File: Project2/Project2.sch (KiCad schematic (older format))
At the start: 75 parts

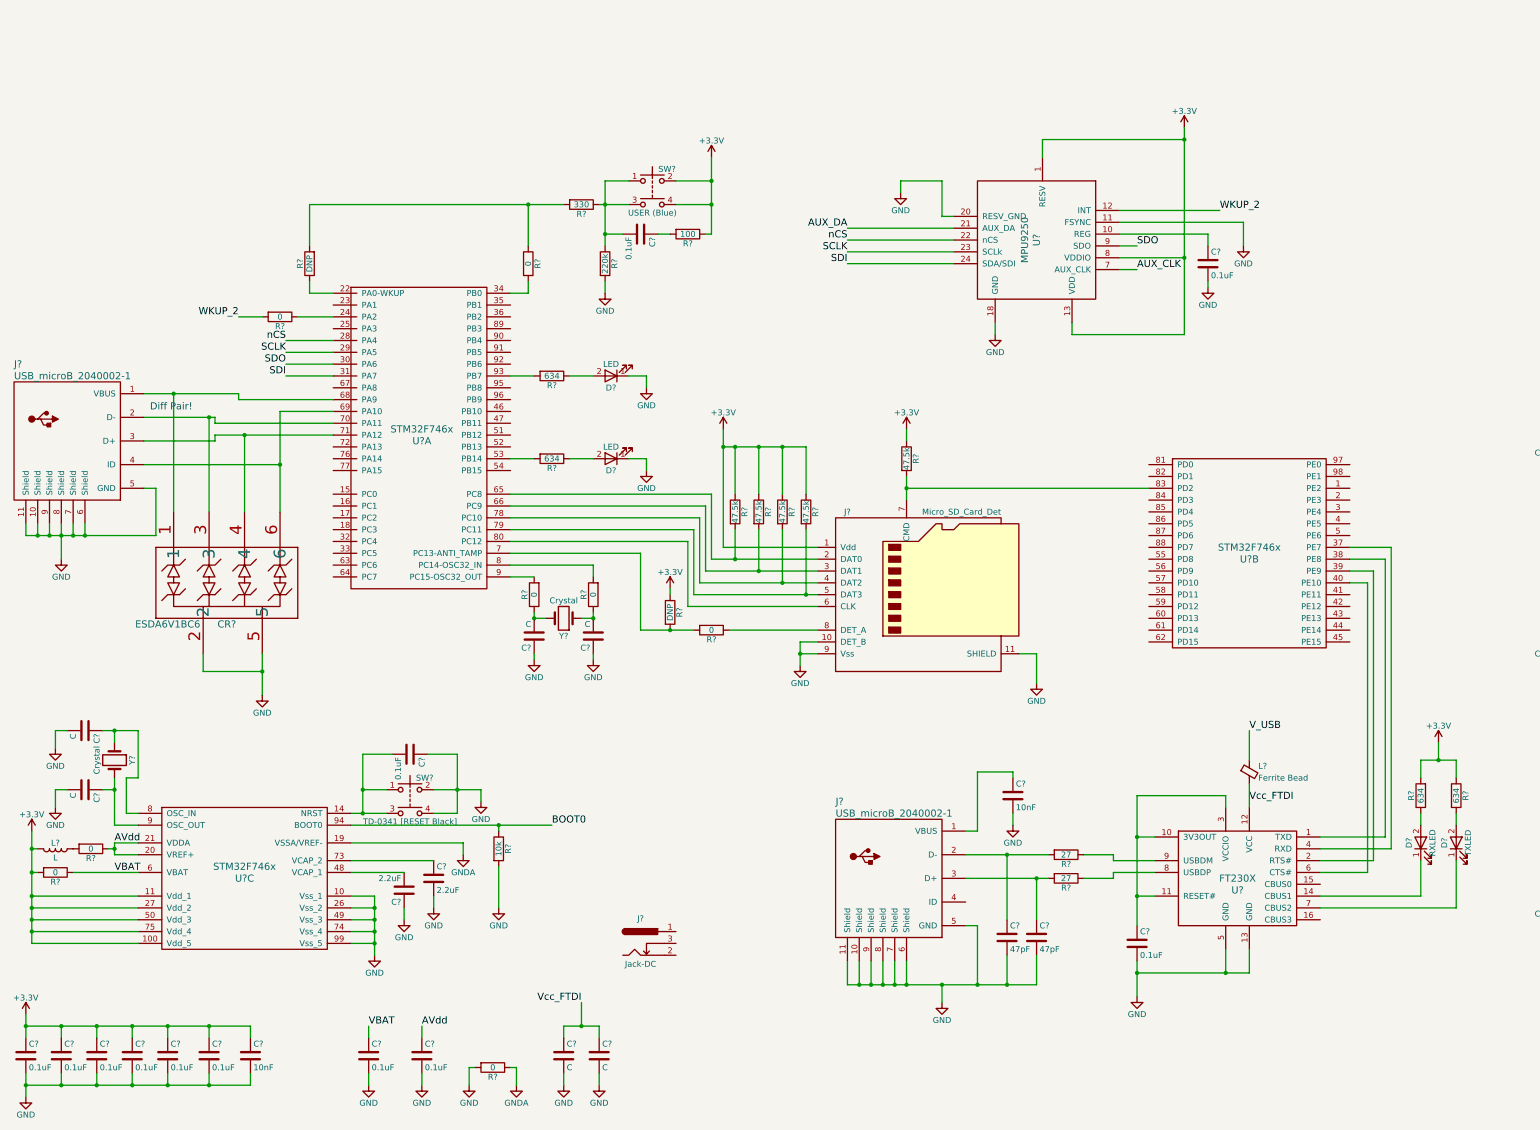
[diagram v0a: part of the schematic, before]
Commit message: Made some updates
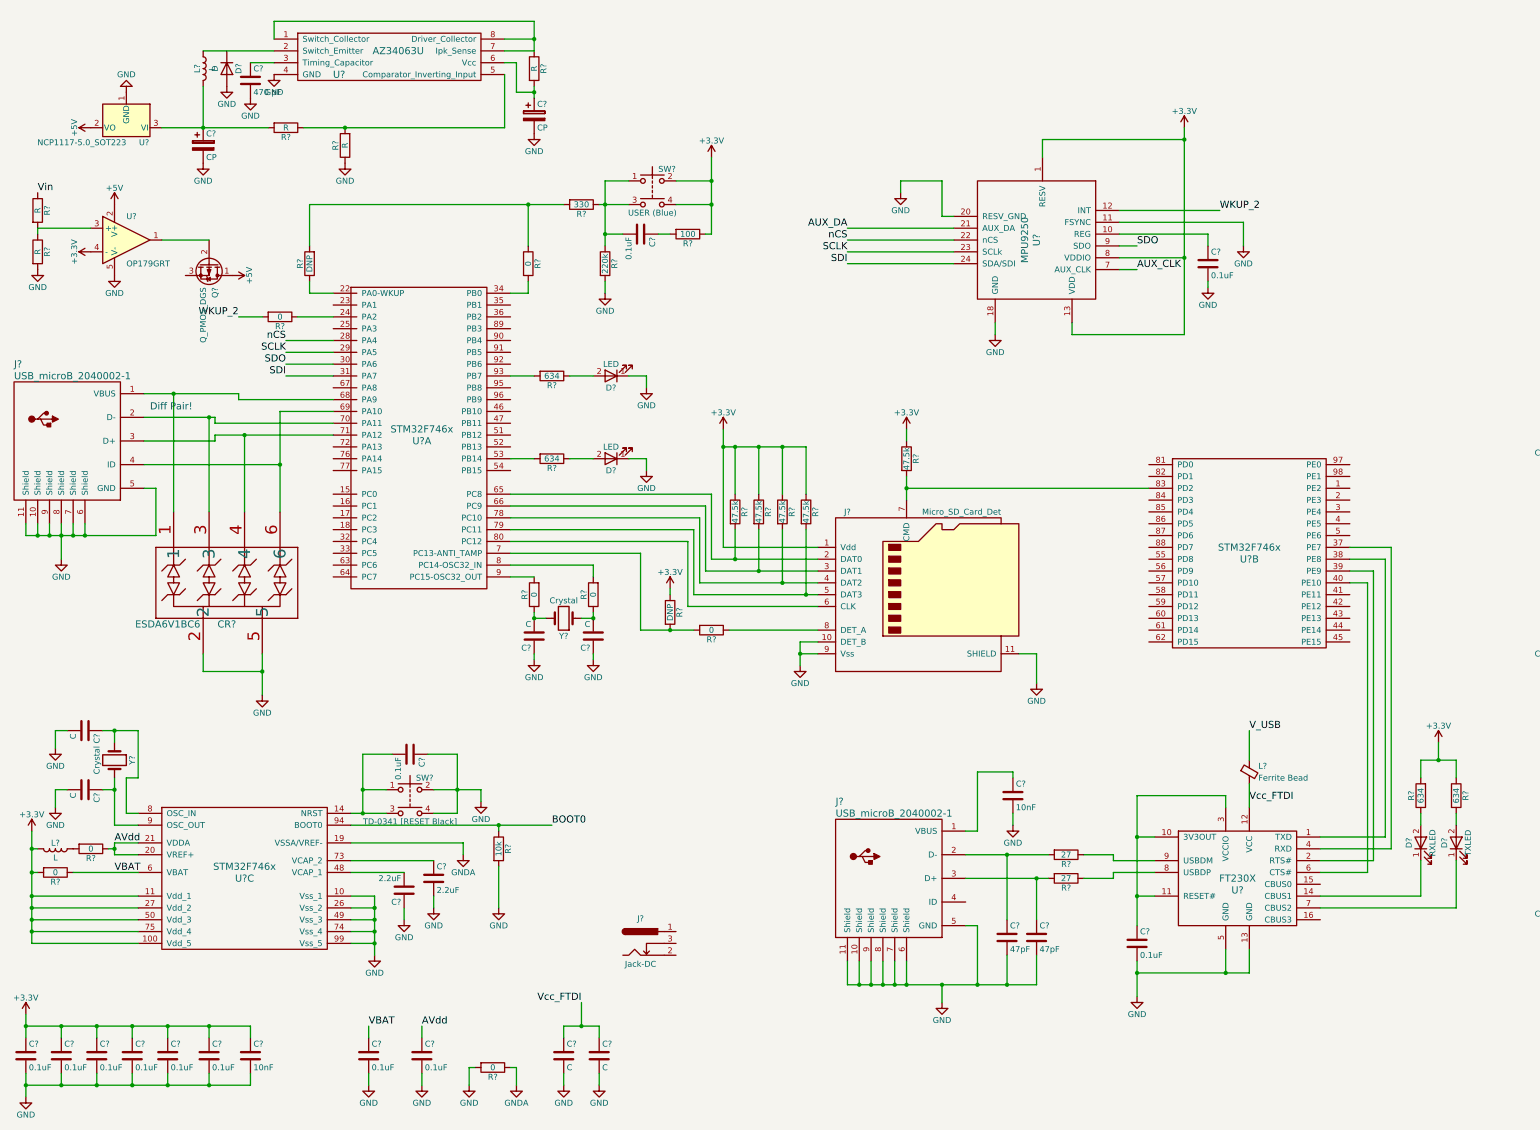
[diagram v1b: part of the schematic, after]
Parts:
- added C?: 470 pF, symbol C
- added C? (x2): CP, symbol CP
- added D?: D, symbol D
- added L?: L, symbol L
- added Q?: Q_PMOS_DGS, symbol Q_PMOS_DGS
- added R? (x5): R, symbol R
- added U?: AZ34063U, symbol AZ34063U
- added U?: NCP1117-5.0_SOT223, TO_SOT_Packages_SMD:SOT-223-3Lead_TabPin2, symbol NCP1117-5.0_SOT223
- added U?: OP179GRT, TO_SOT_Packages_SMD:SOT-23-5, symbol OP179GRT
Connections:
- net +3V3: now also U?.4 (-)
- net GND: now also C?.2, C?.2, C?.2, D?.2 (A), R?.1, R?.2, U?.1 (GND), U?.4 (GND), U?.5 (V-)
- new net: R?.1, U?.1 (Switch_Collector), U?.7 (Ipk_Sense), U?.8 (Driver_Collector)
- new net: L?.1, U?.2 (Switch_Emitter)
- new net: C?.1, U?.3 (Timing_Capacitor)
- new net: R?.1, R?.2, U?.5 (Comparator_Inverting_Input)
- new net: C?.1, R?.2, U?.6 (Vcc)
- new net: C?.1, L?.2, R?.2, U?.3 (VI)
- new net: Q?.2 (G), U?.1
- new net: R?.1, R?.2, U?.3 (+)
- new net +5V: Q?.1 (D), U?.2 (V+), U?.2 (VO)
- new net Vin: R?.1
